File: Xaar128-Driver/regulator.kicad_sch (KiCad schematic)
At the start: 43 parts, among them U11 LM317_TO-220, U13 MCP4725xxx-xCH, U14 ISO1541, U15 L7824, U16 MC78L05_SOT89, U17 TLC272, U18 MCP3021

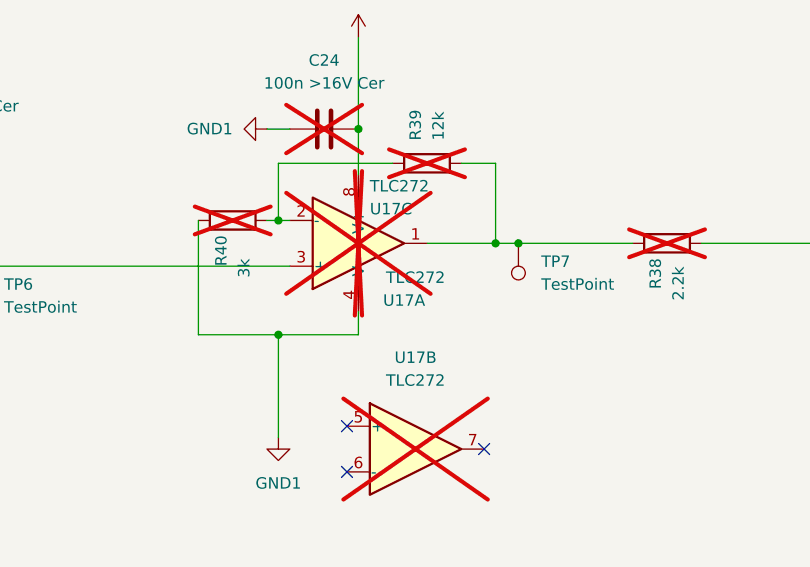
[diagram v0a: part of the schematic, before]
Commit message: switch opv to lm358
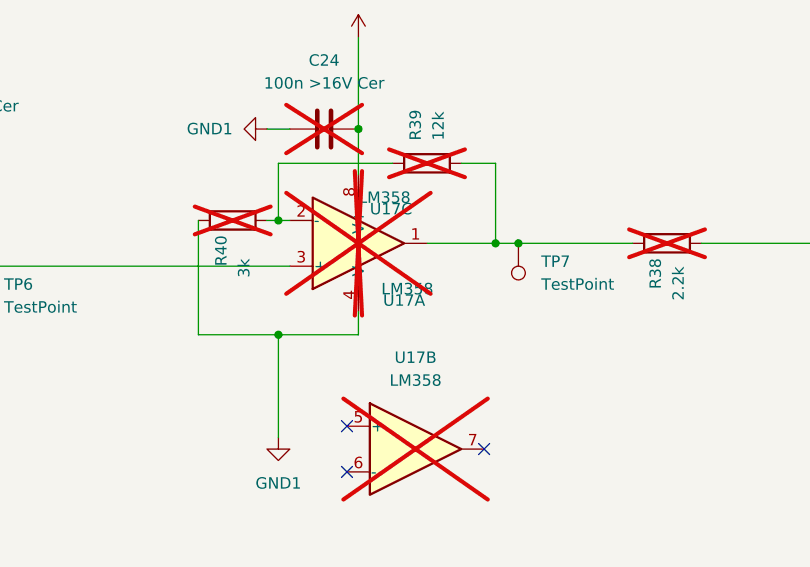
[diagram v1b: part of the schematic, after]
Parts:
- U17: value TLC272 -> LM358; symbol Amplifier_Operational:TLC272 -> Amplifier_Operational:LM358
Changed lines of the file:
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@@
 	(wire
 		(pts
+			(xy 130.81 80.01) (xy 138.43 80.01)
+		)
+		(stroke
+			(width 0)
+			(type default)
+		)
+	)
+	(wire
+		(pts
 			(xy 158.75 33.02) (xy 161.29 33.02)
 		)
@@
 	(wire
 		(pts
-			(xy 130.81 80.01) (xy 138.43 80.01)
-		)
-		(stroke
-			(width 0)
-			(type default)
-		)
-	)
-	(wire
-		(pts
 			(xy 134.62 146.05) (xy 134.62 151.13)
 		)
@@
 	)
 	(symbol
-		(lib_id "Amplifier_Operational:TLC272")
+		(lib_id "Amplifier_Operational:LM358")
 		(at 125.73 80.01 0)
 		(unit 3)
@@
 			)
 		)
-		(property "Value" "TLC272"
-			(at 124.46 73.66 0)
+		(property "Value" "LM358"
+			(at 125.73 85.09 0)
 			(effects
 				(font
@@
 	)
 	(symbol
-		(lib_id "Amplifier_Operational:TLC272")
+		(lib_id "Amplifier_Operational:LM358")
 		(at 123.19 80.01 0)
 		(mirror x)
@@
 			)
 		)
-		(property "Value" "TLC272"
-			(at 129.54 83.82 0)
+		(property "Value" "LM358"
+			(at 123.19 74.93 0)
 			(effects
 				(font
 					(size 1.27 1.27)
 				)
+				(justify left)
 			)
 		)
@@
 	)
 	(symbol
-		(lib_id "Amplifier_Operational:TLC272")
+		(lib_id "Amplifier_Operational:LM358")
 		(at 129.54 102.87 0)
 		(unit 2)
@@
 			)
 		)
-		(property "Value" "TLC272"
+		(property "Value" "LM358"
 			(at 129.54 95.25 0)
 			(effects
